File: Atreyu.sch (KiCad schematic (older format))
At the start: 122 parts, among them SW1 SW_Push, U1 Elite-C

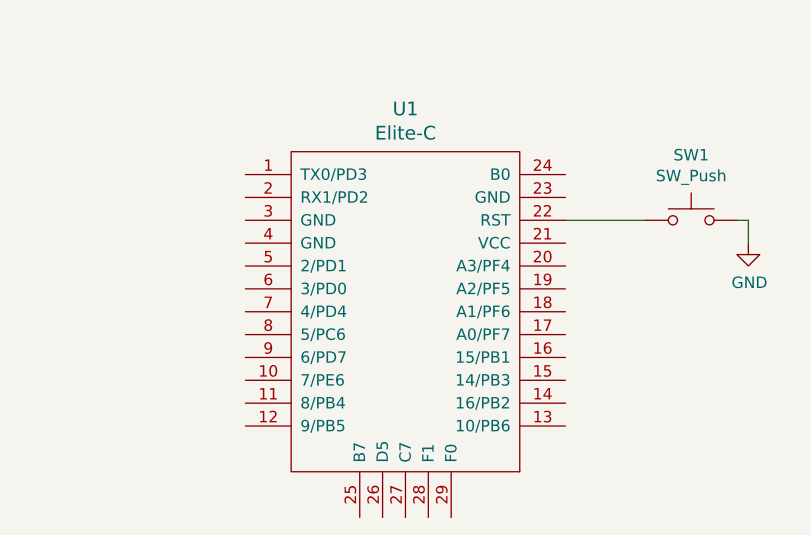
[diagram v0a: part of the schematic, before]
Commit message: PCB initial commit.
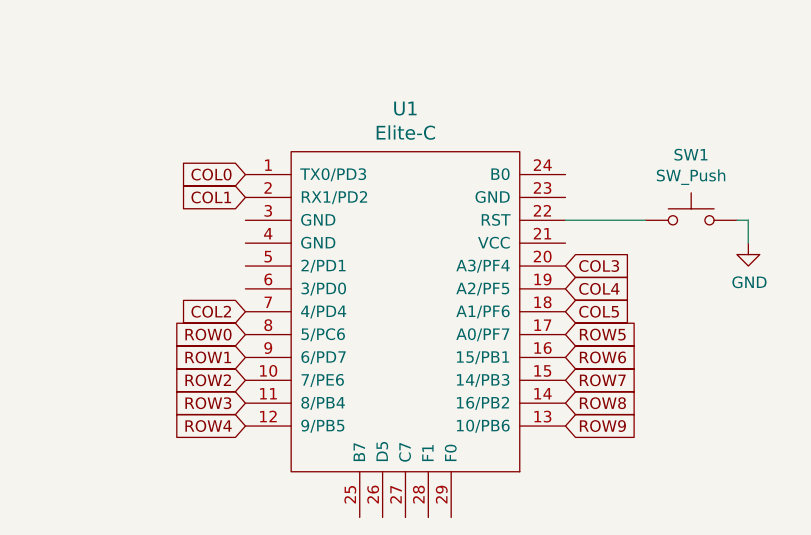
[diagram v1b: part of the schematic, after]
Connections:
- net COL0: now also U1.1 (TX0/PD3)
- net COL1: now also U1.2 (RX1/PD2)
- net COL2: now also U1.7 (4/PD4)
- net COL3: now also U1.20 (A3/PF4)
- net COL4: now also U1.19 (A2/PF5)
- net COL5: now also U1.18 (A1/PF6)
- net ROW0: now also U1.8 (5/PC6)
- net ROW1: now also U1.9 (6/PD7)
- net ROW2: now also U1.10 (7/PE6)
- net ROW3: now also U1.11 (8/PB4)
- net ROW4: now also U1.12 (9/PB5)
- net ROW5: now also U1.17 (A0/PF7)
- net ROW6: now also U1.16 (15/PB1)
- net ROW7: now also U1.15 (14/PB3)
- net ROW8: now also U1.14 (16/PB2)
- net ROW9: now also U1.13 (10/PB6)
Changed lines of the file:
@@
 Text GLabel 4750 1650 0    50   Input ~ 0
 ROW9
+Text GLabel 5250 5850 0    50   Input ~ 0
+COL0
+Text GLabel 5250 5950 0    50   Input ~ 0
+COL1
+Text GLabel 5250 6450 0    50   Input ~ 0
+COL2
+Text GLabel 6650 6250 2    50   Input ~ 0
+COL3
+Text GLabel 6650 6350 2    50   Input ~ 0
+COL4
+Text GLabel 6650 6450 2    50   Input ~ 0
+COL5
+Text GLabel 5250 6550 0    50   Input ~ 0
+ROW0
+Text GLabel 5250 6650 0    50   Input ~ 0
+ROW1
+Text GLabel 5250 6750 0    50   Input ~ 0
+ROW2
+Text GLabel 5250 6850 0    50   Input ~ 0
+ROW3
+Text GLabel 5250 6950 0    50   Input ~ 0
+ROW4
+Text GLabel 6650 6550 2    50   Input ~ 0
+ROW5
+Text GLabel 6650 6650 2    50   Input ~ 0
+ROW6
+Text GLabel 6650 6750 2    50   Input ~ 0
+ROW7
+Text GLabel 6650 6850 2    50   Input ~ 0
+ROW8
+Text GLabel 6650 6950 2    50   Input ~ 0
+ROW9
 $EndSCHEMATC
